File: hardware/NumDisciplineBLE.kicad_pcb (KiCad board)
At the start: 2 copper layers, 22 parts, among them J1 Conn_02x20_Counter_Clockwise, J2 SWD, J3 Ex_Bat, J4 Ex_USB, Q1 AO3407, Q2 AO3407, U1 E73-2G4M08S1C, U2 XC6220B331MR-G, U3 TP4054, X1 32.768kHz

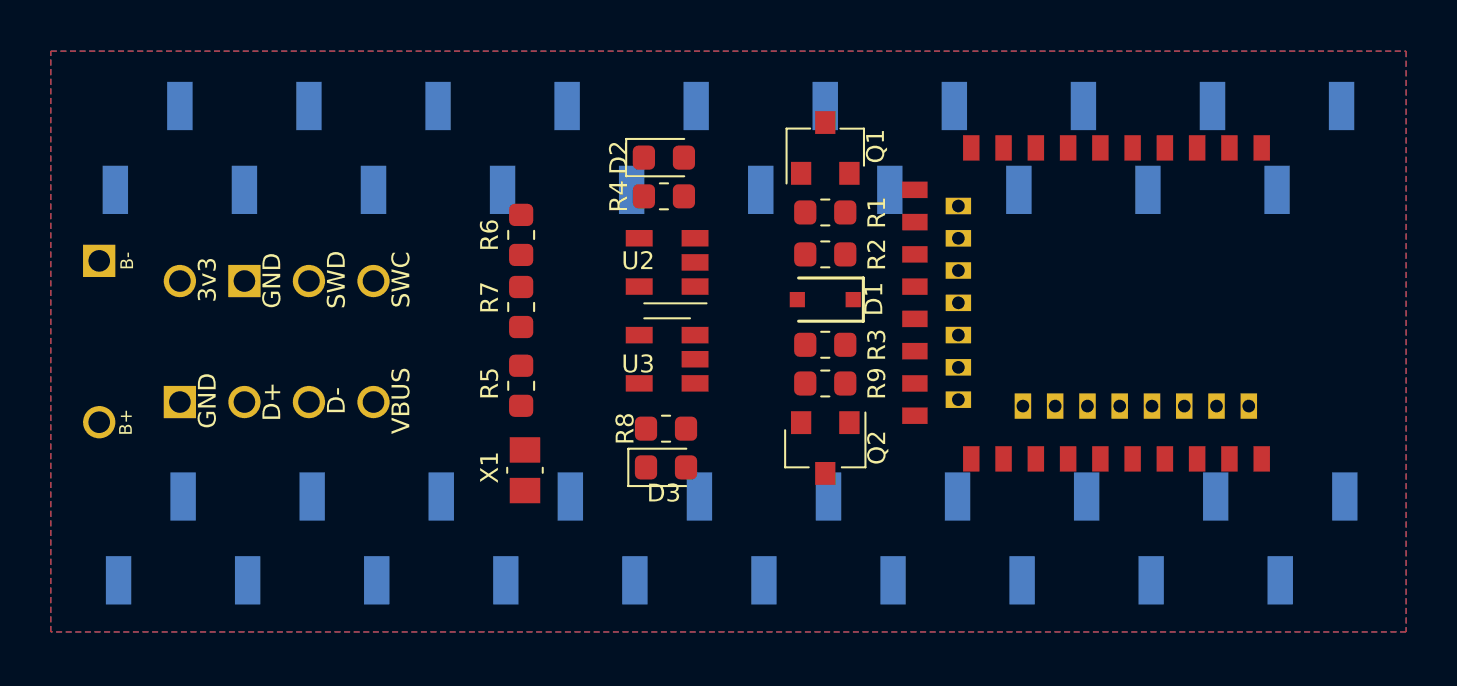
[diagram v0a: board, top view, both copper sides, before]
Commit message: pre-routing2
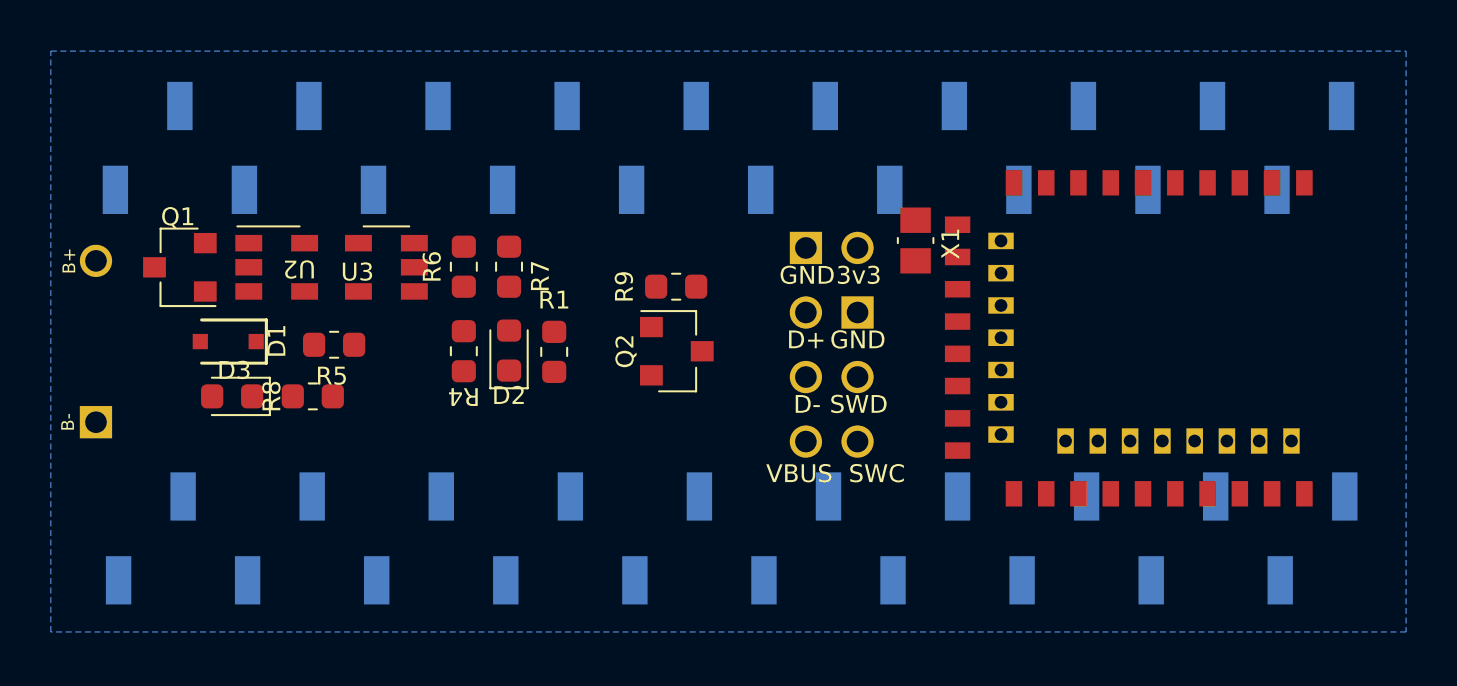
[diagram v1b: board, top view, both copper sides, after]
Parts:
- removed R2, R3: 5.1K, Resistor_SMD:R_0603_1608Metric
- moved J2 26.7 mm to (124.5, 35.1), turned to 180 degrees
- moved Q1 25.8 mm to (97.8, 35.8), turned to 180 degrees
- moved J4 25.4 mm to (122.4, 35.1), turned to 180 degrees
- moved D1 23.6 mm to (99.7, 38.7)
- moved X1 17.8 mm to (126.7, 34.8), turned to 90 degrees
- moved D3 17.3 mm to (99.8, 40.9), turned to 180 degrees
- moved U2 15.4 mm to (101.6, 35.8), turned to 0 degrees
- moved R8 14.0 mm to (103.0, 40.9)
- moved R1 12.0 mm to (112.5, 39.1), turned to 270 degrees
- moved U3 11.6 mm to (105.9, 35.8)
- moved R4 9.96 mm to (109.0, 39.1), turned to 90 degrees
- moved D2 9.74 mm to (110.7, 39.1), turned to 90 degrees
- moved R5 7.54 mm to (103.9, 38.9), turned to 180 degrees
- moved R9 7.00 mm to (117.3, 36.6), turned to 0 degrees
- moved Q2 6.97 mm to (117.3, 39.1), turned to 0 degrees
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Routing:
- removed copper zone on F.Cu, net GND

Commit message: post-autoroute
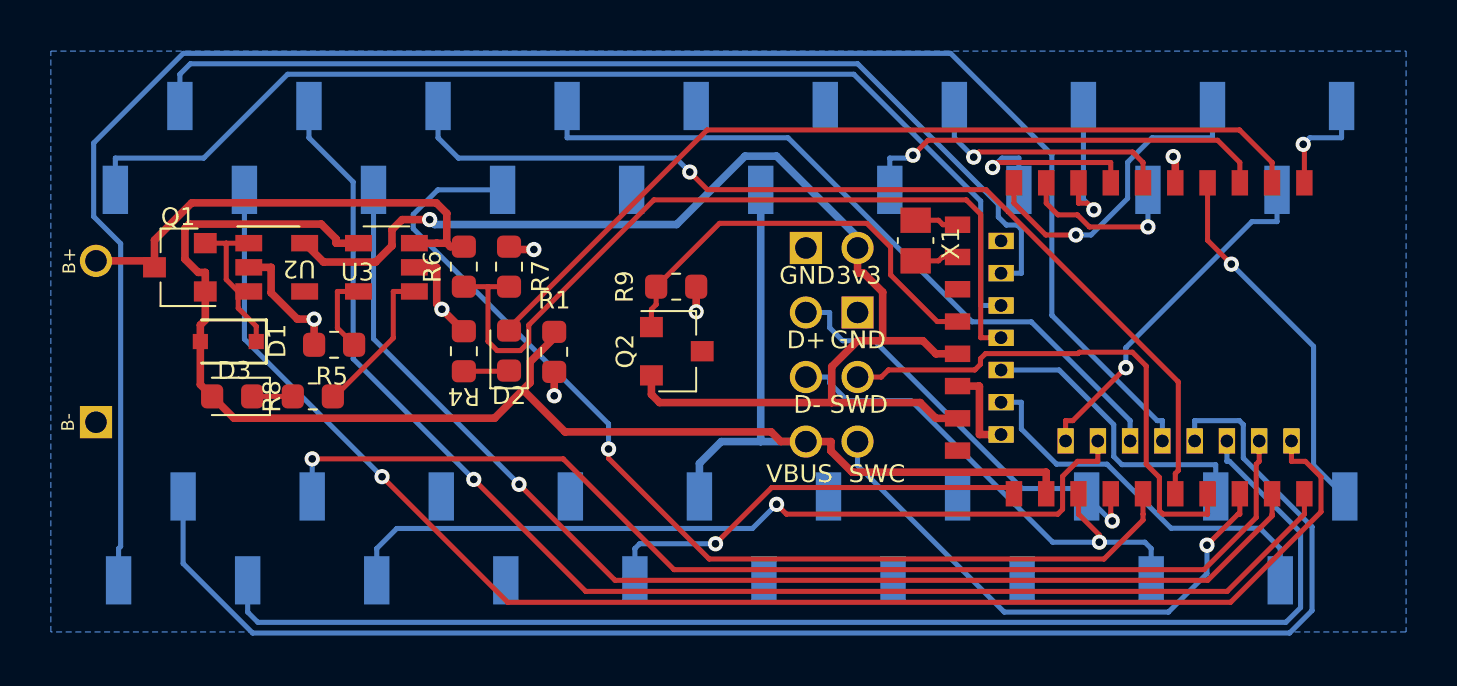
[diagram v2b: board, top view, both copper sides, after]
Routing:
- net /P0.22: track 0.00 -> 71.7 mm
- net VBUS: track 0.00 -> 69.3 mm
- net /P1.00: track 0.00 -> 59.8 mm
- net /P1.06: track 0.00 -> 57.6 mm, vias 0 -> 1
- net /P0.10: track 0.00 -> 54.0 mm, vias 0 -> 1
- net /P1.02: track 0.00 -> 50.9 mm
- net nRF_VDD: track 0.00 -> 50.5 mm, vias 0 -> 1
- net /P0.09: track 0.00 -> 47.1 mm, vias 0 -> 1
- net /P1.04: track 0.00 -> 44.3 mm, vias 0 -> 1
- net /P0.08: track 0.00 -> 43.6 mm
- net /P0.13: track 0.00 -> 41.0 mm, vias 0 -> 1
- net /P0.06: track 0.00 -> 40.1 mm
- net /P0.24: track 0.00 -> 38.8 mm, vias 0 -> 1
- net BLUE_LED: track 0.00 -> 34.7 mm
- net /P0.17: track 0.00 -> 32.9 mm, vias 0 -> 1
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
